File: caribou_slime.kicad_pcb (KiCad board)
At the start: 2 copper layers, 36.1 x 28.4 mm, 11 parts, among them J1 Conn_01x02_MountingPin, U1 ESP32-C3_SUPERMINI, U2 BMI270

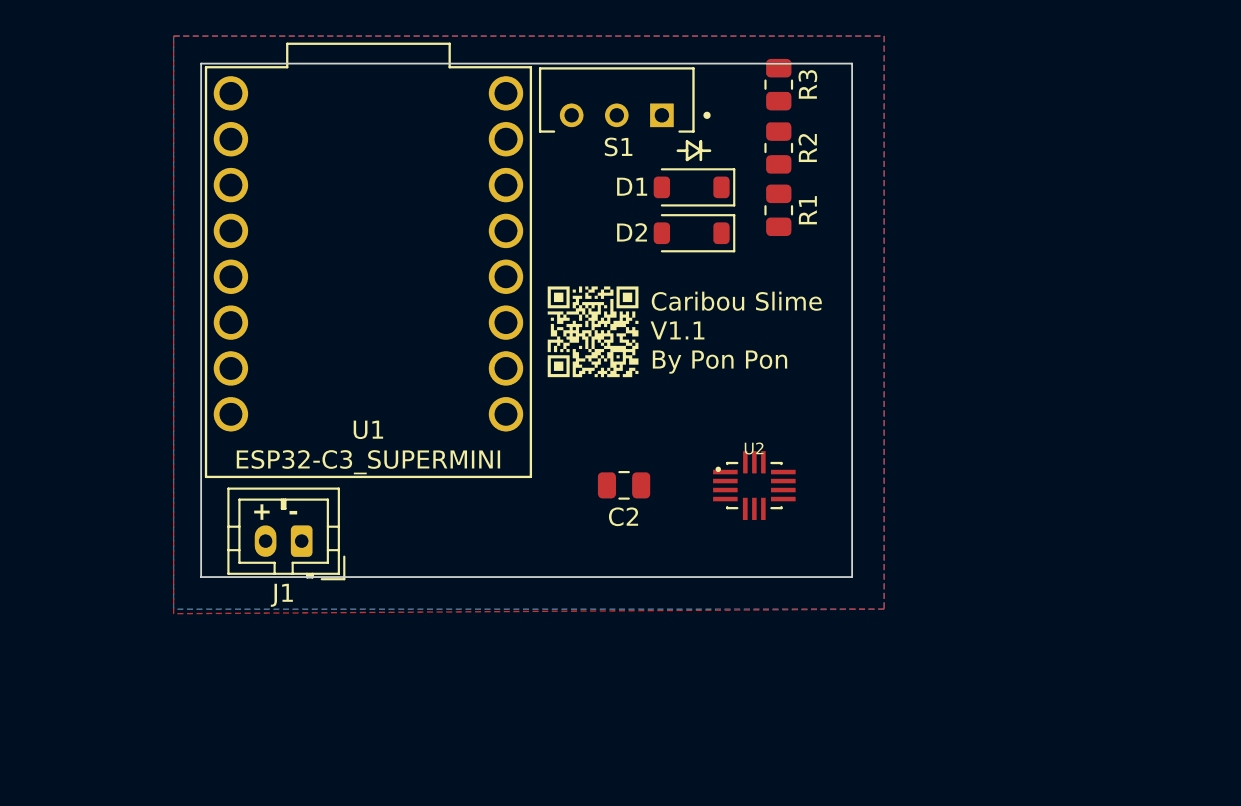
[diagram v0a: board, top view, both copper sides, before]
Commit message: refactor(pcb): Design V1 PCB for Hyperion
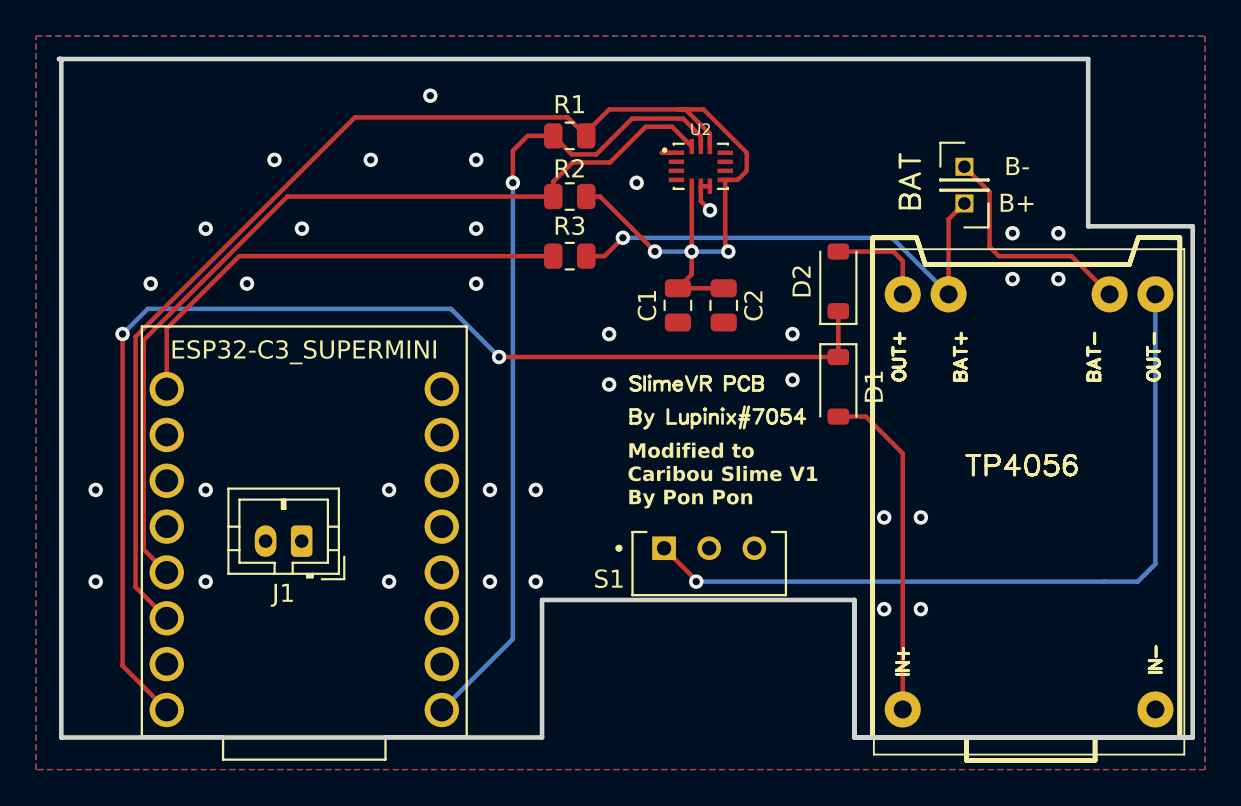
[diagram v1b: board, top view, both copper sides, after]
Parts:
- removed G***: LOGO, LOGO
- added C1: 100nF, Capacitor_SMD:C_0805_2012Metric, F.Cu at (59.7, 39.0)
- added H1: B+, Connector_PinHeader_2.54mm:PinHeader_1x01_P2.54mm_Vertical, F.Cu at (75.6, 33.4)
- added H2: B-, Connector_PinHeader_2.54mm:PinHeader_1x01_P2.54mm_Vertical, F.Cu at (75.6, 31.4)
- added U3: TP4056, TP4056_Charging_Board:TP4056 Charging Board, F.Cu at (87.7, 63.9)
- moved S1 24.5 mm to (61.4, 52.5), turned to 0 degrees
- moved U2 17.9 mm to (61.0, 31.3)
- moved R3 15.0 mm to (53.7, 36.3), turned to 0 degrees
- moved U1 14.8 mm to (39.0, 51.6), turned to 180 degrees
- moved D1 13.7 mm to (68.6, 43.6), turned to -90 degrees
- moved R1 12.3 mm to (53.7, 29.7), turned to 180 degrees
- moved R2 11.9 mm to (53.7, 33.0), turned to 180 degrees
- moved C2 11.4 mm to (62.2, 39.0), turned to -90 degrees
- moved D2 8.55 mm to (68.6, 37.7), turned to 90 degrees
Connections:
- R3 pad 2: /B+ -> Net-(U3-B+)
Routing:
- net +3V3: track 0.00 -> 84.6 mm, vias 0 -> 3
- net +5V: track 0.00 -> 65.7 mm, vias 0 -> 2
- net Net-(U3-OUT-): track 0.00 -> 49.6 mm
- net SDA: track 0.00 -> 45.6 mm, vias 0 -> 1
- net /B+: track 0.00 -> 43.4 mm, vias 0 -> 1
- net unconnected-(U2-ASDX-Pad2): track 0.00 -> 27.2 mm, vias 0 -> 1
- net unconnected-(S1-Pad3): track 0.00 -> 26.4 mm
- net Net-(D1-A): track 0.00 -> 18.6 mm
- net unconnected-(U2-INT2-Pad9): track 0.00 -> 12.8 mm
- net Net-(D2-A): track 0.00 -> 5.63 mm
- net GND: track 0.00 -> 3.23 mm, vias 0 -> 34
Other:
- board size 36.1 x 28.4 mm -> 62.8 x 37.6 mm
- board text added: "Modified to Caribou Slime V1 By Pon Pon"
- board text removed: "+"
- board text removed: "-"
- board text removed: "Caribou Slime V1.1 By Pon Pon"
